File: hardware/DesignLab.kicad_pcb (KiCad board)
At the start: 2 copper layers, 87 parts, among them J1 Micro_SD_Card_Det, J2 Conn_01x04_Female, P1 USB_C_Plug_USB2.0, Q1 DMG3415U-7, SW1 SW_DPDT_x2, SW10 Button, SW11 Button, SW12 RESET, SW13 ON, SW14 VOL, SW15 BOOT, SW2 SW_DPDT_x2, SW3 REC, SW4 Button, SW5 Button, SW6 Button, SW7 Button, SW8 Button, SW9 Button, U1 SPH0641LM4H, U10 MCP4018-xxxxLT, U2 RP2040, U3 QRE1113, U4 QRE1113, U5 QRE1113, U6 AT25SF128A, U7 PAM8302AAD, U8 AP2112K-3.3, U9 QRE1113, Y1 12Mhz

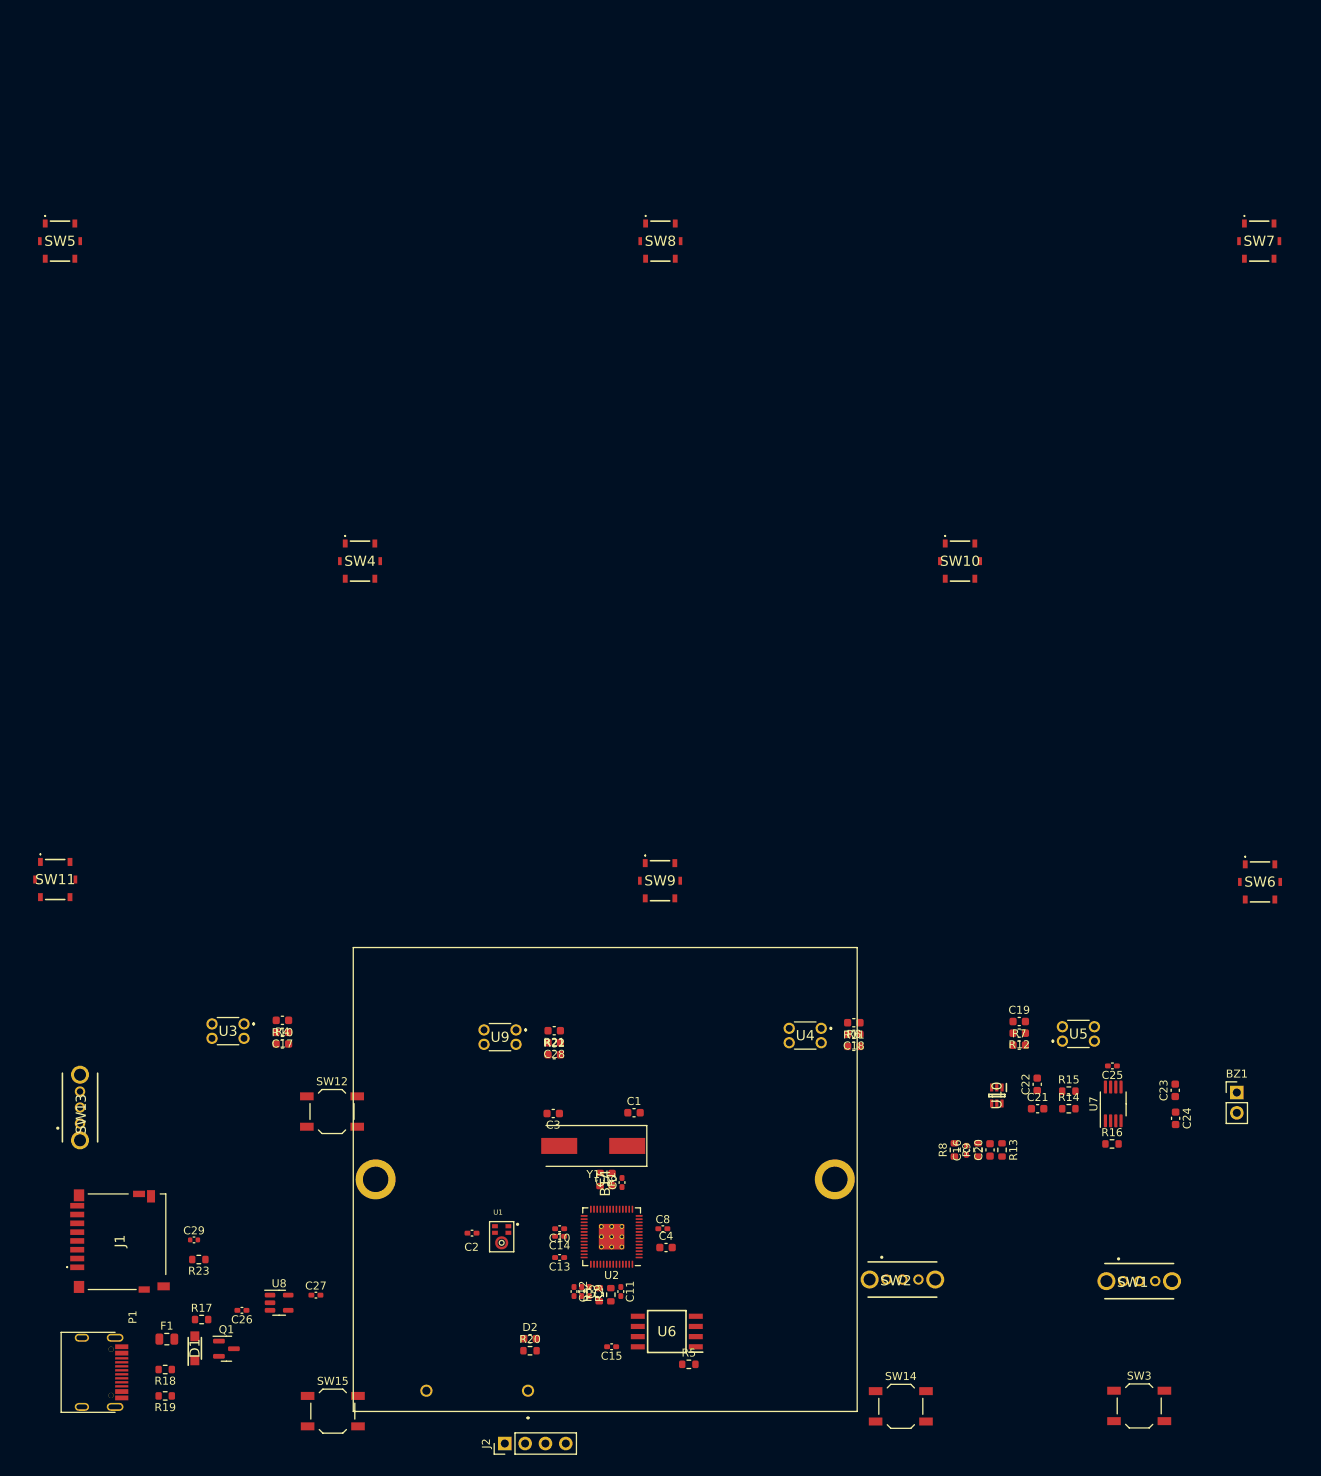
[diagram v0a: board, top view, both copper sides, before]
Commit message: More PCB design proposal
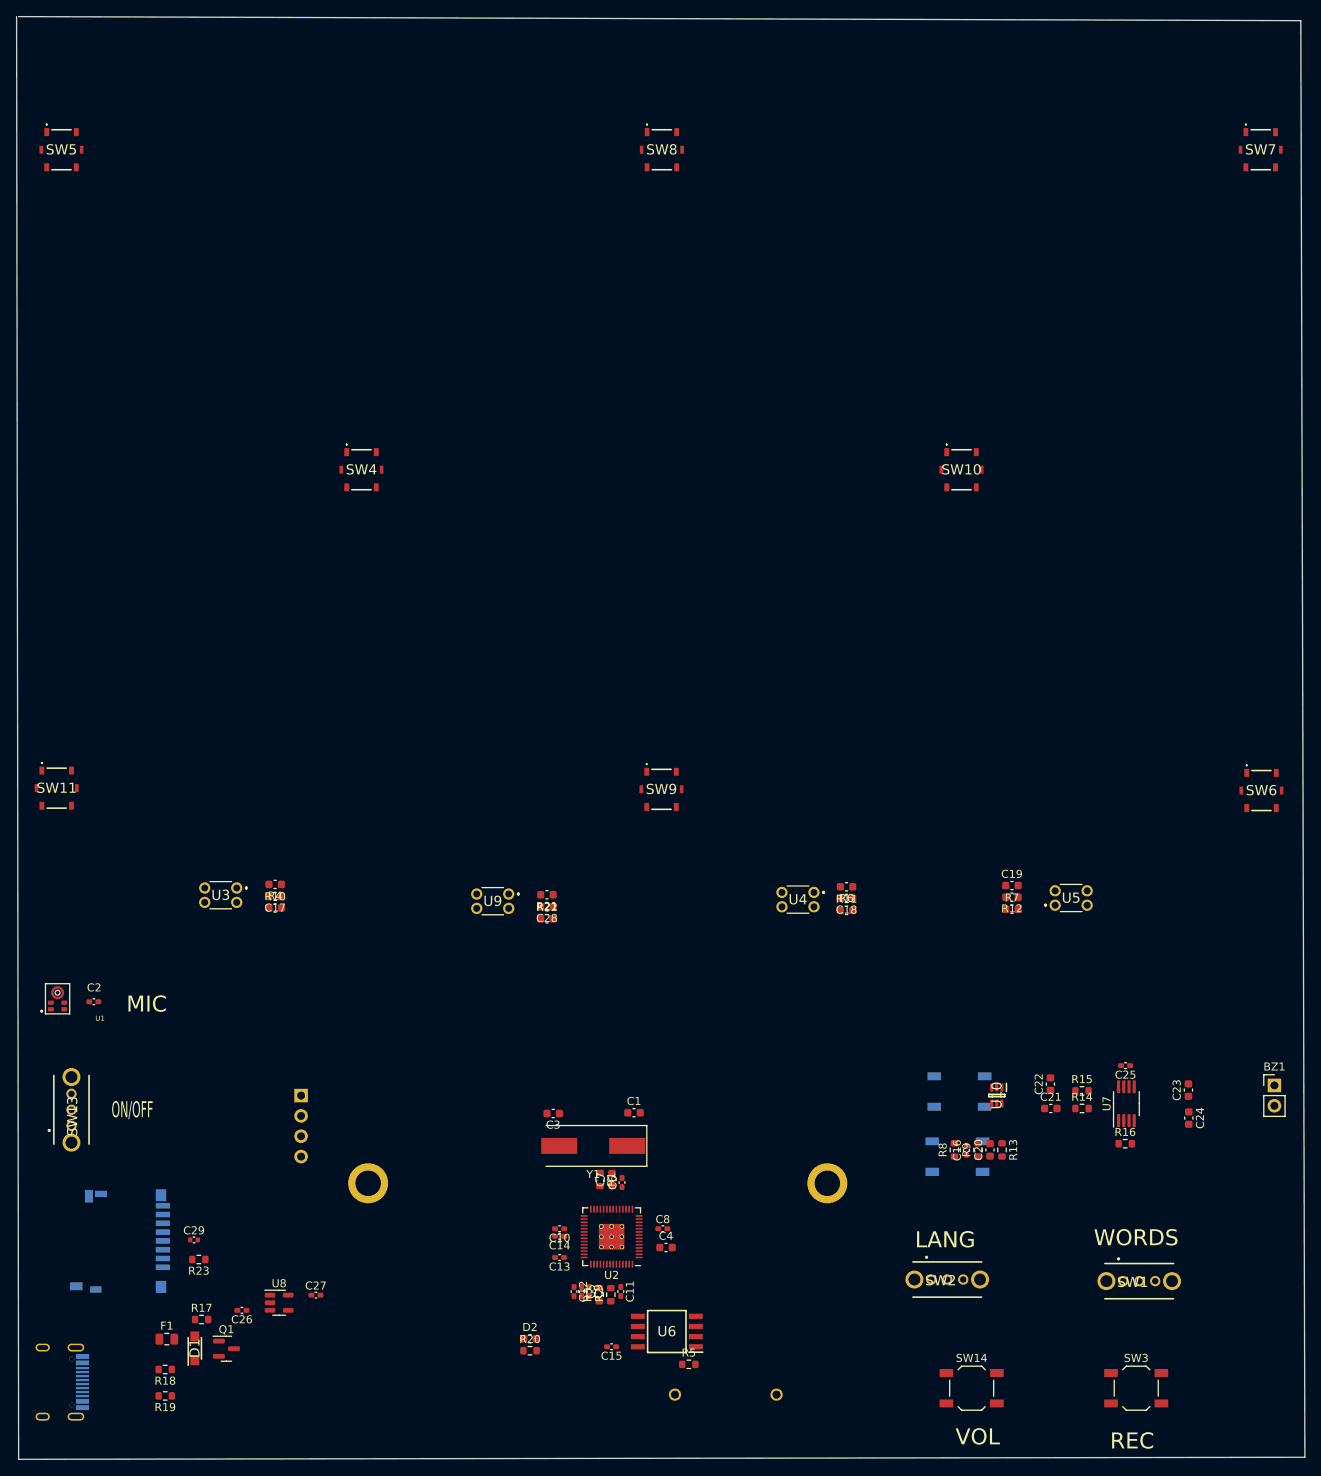
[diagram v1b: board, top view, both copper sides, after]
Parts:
- BT4, J1, J2, P1, SW12, SW15: moved to B.Cu
- moved SW15 87.9 mm to (236.7, 165.1), turned to 180 degrees
- moved SW12 78.4 mm to (236.5, 173.2), turned to 180 degrees
- moved U1 63.7 mm to (124.0, 152.7), turned to 180 degrees
- moved C2 55.4 mm to (128.5, 153.9), turned to 0 degrees
- moved J2 50.4 mm to (154.4, 165.6), turned to 180 degrees
- moved BT4 18.4 mm to (201.2, 203.0)
- moved C28 17.0 mm to (185.2, 142.0)
- moved R10 17.0 mm to (151.2, 142.2)
- moved R12 17.0 mm to (243.3, 140.8)
- moved R21 17.0 mm to (185.2, 140.5)
- moved R22 17.0 mm to (185.2, 143.5)
- moved R6 17.0 mm to (222.6, 139.5)
- moved R7 17.0 mm to (243.3, 142.3)
- moved U3 17.0 mm to (146.4, 139.7)
- moved U5 17.0 mm to (248.7, 141.8)
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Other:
- board outline added: 161 x 180.3 mm
- board text added: "LANG"
- board text added: "MIC"
- board text added: "ON/OFF"
- board text added: "REC"
- board text added: "VOL"
- board text added: "WORDS"
